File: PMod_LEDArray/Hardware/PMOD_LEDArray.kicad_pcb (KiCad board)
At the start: 2 copper layers, 81.6 x 23 mm, 133 parts, among them J1 Conn_02x06_Odd_Even, U1 GN1640

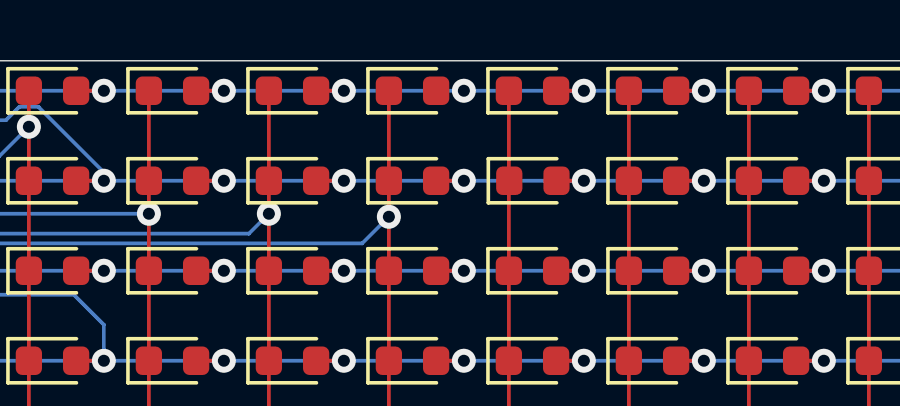
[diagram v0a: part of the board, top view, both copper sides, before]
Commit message: Fix missing connecting track
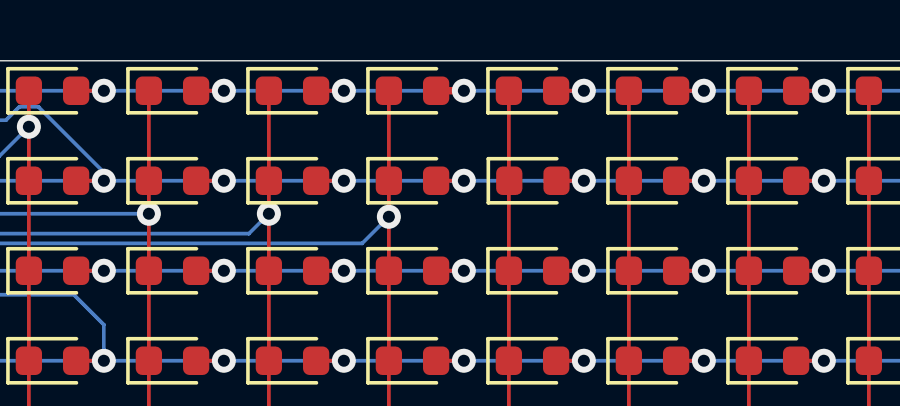
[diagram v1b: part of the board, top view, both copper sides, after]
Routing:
- net /SEG8: track 94.8 -> 95.7 mm
